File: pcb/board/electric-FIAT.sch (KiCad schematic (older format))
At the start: 25 parts, among them J1 Conn_01x10_Female, U4 OPA356xxDBV, U5 OPA356xxDBV, U6 STM32F405RGTx

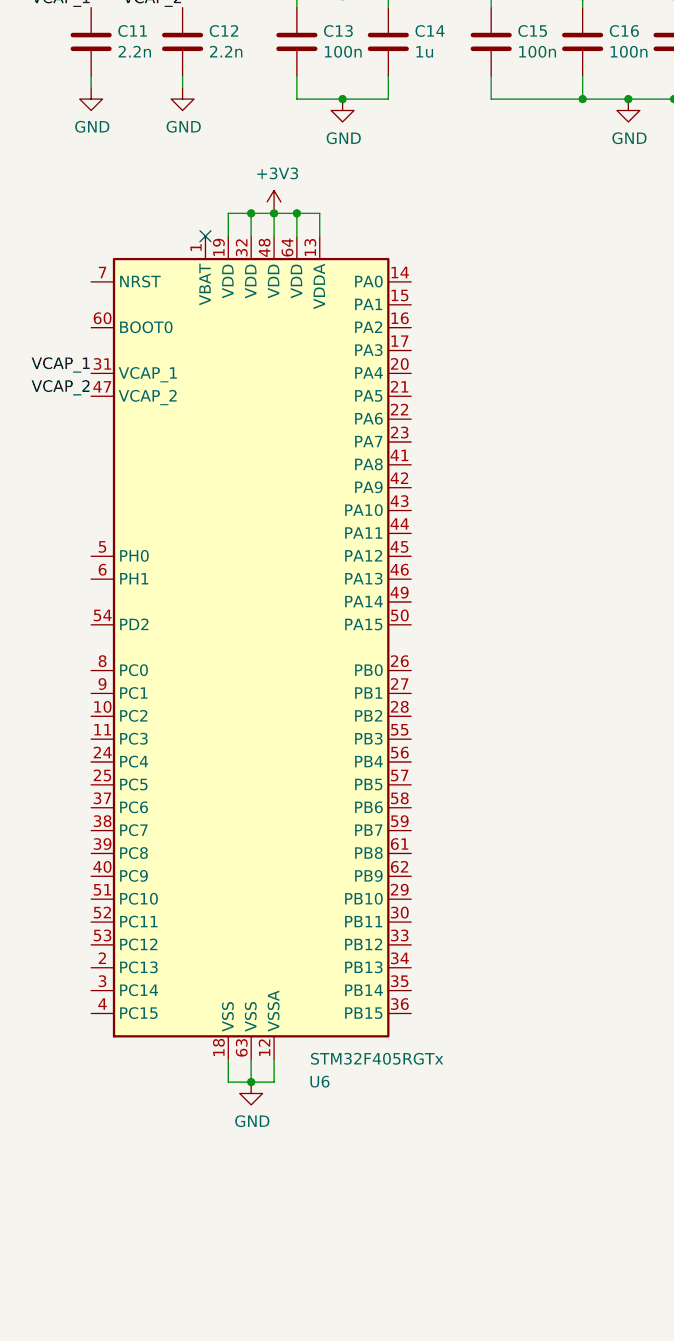
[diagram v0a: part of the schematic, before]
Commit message: Initialized STM32F405RGTx
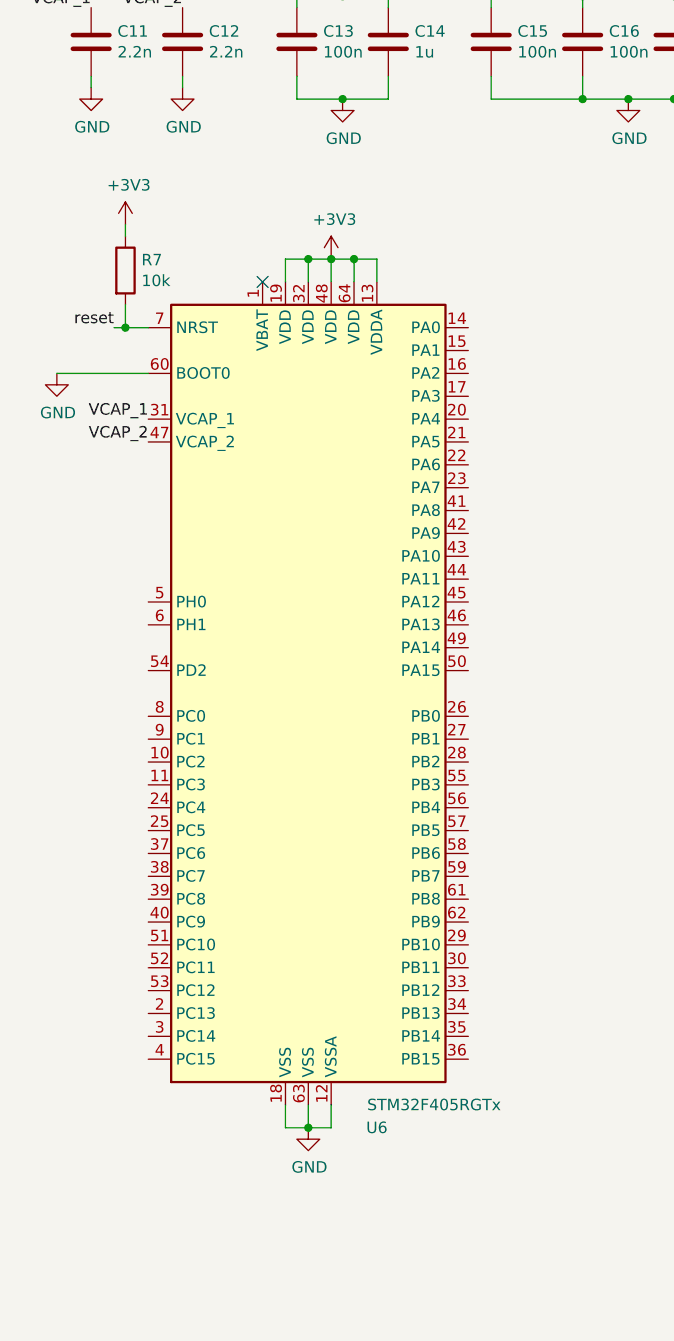
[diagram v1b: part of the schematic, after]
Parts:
- added R7: 10k, Resistor_SMD:R_0805_2012Metric, symbol Device:R
- J1: footprint (none) -> Connector_PinSocket_2.54mm:PinSocket_1x10_P2.54mm_Vertical
- TH1, TH2: footprint (none) -> TerminalBlock_RND:TerminalBlock_RND_205-00012_1x02_P5.00mm_Horizontal
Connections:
- net +3V3: now also R7.1
- net GND: now also U6.60 (BOOT0)
- net reset: now reaches U6.7 (NRST)
- net reset: now also R7.2
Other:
- moved on the sheet: U6
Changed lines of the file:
@@
 F 0 "TH1" H 7247 1746 50  0000 L CNN
 F 1 "KTY81" H 7247 1655 50  0000 L CNN
-F 2 "" V 7350 1700 50  0001 C CNN
+F 2 "TerminalBlock_RND:TerminalBlock_RND_205-00012_1x02_P5.00mm_Horizontal" V 7350 1700 50  0001 C CNN
 F 3 "http://www.nxp.com/documents/data_sheet/KTY81_SER.pdf" H 7150 1650 50  0001 C CNN
 	1    7150 1700
@@
 F 0 "TH2" H 9198 1746 50  0000 L CNN
 F 1 "Thermistor_NTC" H 9198 1655 50  0000 L CNN
-F 2 "" H 9100 1750 50  0001 C CNN
+F 2 "TerminalBlock_RND:TerminalBlock_RND_205-00012_1x02_P5.00mm_Horizontal" H 9100 1750 50  0001 C CNN
 F 3 "~" H 9100 1750 50  0001 C CNN
 	1    9100 1700
@@
 L MCU_ST_STM32F4:STM32F405RGTx U6
 U 1 1 5DC72DB0
-P 1550 3900
-F 0 "U6" H 1850 2000 50  0000 C CNN
-F 1 "STM32F405RGTx" H 2100 2100 50  0000 C CNN
-F 2 "Package_QFP:LQFP-64_10x10mm_P0.5mm" H 950 2200 50  0001 R CNN
-F 3 "http://www.st.com/st-web-ui/static/active/en/resource/technical/document/datasheet/DM00037051.pdf" H 1550 3900 50  0001 C CNN
-	1    1550 3900
+P 1800 4100
+F 0 "U6" H 2100 2200 50  0000 C CNN
+F 1 "STM32F405RGTx" H 2350 2300 50  0000 C CNN
+F 2 "Package_QFP:LQFP-64_10x10mm_P0.5mm" H 1200 2400 50  0001 R CNN
+F 3 "http://www.st.com/st-web-ui/static/active/en/resource/technical/document/datasheet/DM00037051.pdf" H 1800 4100 50  0001 C CNN
+	1    1800 4100
 	1    0    0    -1
 $EndComp
@@
 $EndComp
 Wire Wire Line
-	1550 2000 1450 2000
-Wire Wire Line
-	1550 2000 1550 2100
-Connection ~ 1550 2000
-Wire Wire Line
-	1450 2000 1450 2100
-Wire Wire Line
-	1650 2100 1650 2000
-Wire Wire Line
-	1650 2000 1550 2000
-Wire Wire Line
-	1750 2100 1750 2000
-Wire Wire Line
-	1750 2000 1650 2000
-Connection ~ 1650 2000
-Wire Wire Line
-	1850 2100 1850 2000
-Wire Wire Line
-	1850 2000 1750 2000
-Connection ~ 1750 2000
+	1800 2200 1700 2200
+Wire Wire Line
+	1800 2200 1800 2300
+Connection ~ 1800 2200
+Wire Wire Line
+	1700 2200 1700 2300
+Wire Wire Line
+	1900 2300 1900 2200
+Wire Wire Line
+	1900 2200 1800 2200
+Wire Wire Line
+	2000 2300 2000 2200
+Wire Wire Line
+	2000 2200 1900 2200
+Connection ~ 1900 2200
+Wire Wire Line
+	2100 2300 2100 2200
+Wire Wire Line
+	2100 2200 2000 2200
+Connection ~ 2000 2200
 $Comp
 L power:GND #PWR027
 U 1 1 5DC7D7B5
-P 1550 5800
-F 0 "#PWR027" H 1550 5550 50  0001 C CNN
-F 1 "GND" H 1555 5627 50  0000 C CNN
-F 2 "" H 1550 5800 50  0001 C CNN
-F 3 "" H 1550 5800 50  0001 C CNN
-	1    1550 5800
-	1    0    0    -1
-$EndComp
-Wire Wire Line
-	1550 5800 1450 5800
-Wire Wire Line
-	1450 5800 1450 5700
-Wire Wire Line
-	1550 5700 1550 5800
-Connection ~ 1550 5800
-Wire Wire Line
-	1650 5700 1650 5800
-Wire Wire Line
-	1650 5800 1550 5800
+P 1800 6000
+F 0 "#PWR027" H 1800 5750 50  0001 C CNN
+F 1 "GND" H 1805 5827 50  0000 C CNN
+F 2 "" H 1800 6000 50  0001 C CNN
+F 3 "" H 1800 6000 50  0001 C CNN
+	1    1800 6000
+	1    0    0    -1
+$EndComp
+Wire Wire Line
+	1800 6000 1700 6000
+Wire Wire Line
+	1700 6000 1700 5900
+Wire Wire Line
+	1800 5900 1800 6000
+Connection ~ 1800 6000
+Wire Wire Line
+	1900 5900 1900 6000
+Wire Wire Line
+	1900 6000 1800 6000
 $Comp
 L Device:C C12
@@
 	1    0    0    -1
 $EndComp
-Text Label 850  2700 2    50   ~ 0
+Text Label 1100 2900 2    50   ~ 0
 VCAP_1
-Text Label 850  2800 2    50   ~ 0
+Text Label 1100 3000 2    50   ~ 0
 VCAP_2
 Text Label 850  1100 2    50   ~ 0
@@
 Text Notes 1700 1000 0    50   ~ 0
 ADC
-NoConn ~ 1350 2100
+NoConn ~ 1600 2300
 $Comp
 L Device:C C15
@@
 L power:+3V3 #PWR034
 U 1 1 5DCEBEA8
-P 1650 2000
-F 0 "#PWR034" H 1650 1850 50  0001 C CNN
-F 1 "+3V3" H 1665 2173 50  0000 C CNN
-F 2 "" H 1650 2000 50  0001 C CNN
-F 3 "" H 1650 2000 50  0001 C CNN
-	1    1650 2000
+P 1900 2200
+F 0 "#PWR034" H 1900 2050 50  0001 C CNN
+F 1 "+3V3" H 1915 2373 50  0000 C CNN
+F 2 "" H 1900 2200 50  0001 C CNN
+F 3 "" H 1900 2200 50  0001 C CNN
+	1    1900 2200
 	1    0    0    -1
 $EndComp
@@
 F 0 "J1" H 6028 6976 50  0000 L CNN
 F 1 "Conn_01x10_Female" H 6028 6885 50  0000 L CNN
-F 2 "" H 6000 7000 50  0001 C CNN
+F 2 "Connector_PinSocket_2.54mm:PinSocket_1x10_P2.54mm_Vertical" H 6000 7000 50  0001 C CNN
 F 3 "~" H 6000 7000 50  0001 C CNN
 	1    6000 7000
@@
 	5100 6700 5800 6700
 Connection ~ 5100 7000
+$Comp
+L power:GND #PWR041
+U 1 1 5DD53313
+P 700 2700
+F 0 "#PWR041" H 700 2450 50  0001 C CNN
+F 1 "GND" H 705 2527 50  0000 C CNN
+F 2 "" H 700 2700 50  0001 C CNN
+F 3 "" H 700 2700 50  0001 C CNN
+	1    700  2700
+	1    0    0    -1
+$EndComp
+Wire Wire Line
+	700  2700 1100 2700
+Text Label 950  2500 2    50   ~ 0
+reset
+$Comp
+L power:+3V3 #PWR040
+U 1 1 5DD5B29D
+P 1000 2050
+F 0 "#PWR040" H 1000 1900 50  0001 C CNN
+F 1 "+3V3" H 1015 2223 50  0000 C CNN
+F 2 "" H 1000 2050 50  0001 C CNN
+F 3 "" H 1000 2050 50  0001 C CNN
+	1    1000 2050
+	1    0    0    -1
+$EndComp
+$Comp
+L Device:R R7
+U 1 1 5DD5BE82
+P 1000 2250
+F 0 "R7" H 1070 2296 50  0000 L CNN
+F 1 "10k" H 1070 2205 50  0000 L CNN
+F 2 "Resistor_SMD:R_0805_2012Metric" V 930 2250 50  0001 C CNN
+F 3 "~" H 1000 2250 50  0001 C CNN
+	1    1000 2250
+	1    0    0    -1
+$EndComp
+Wire Wire Line
+	1000 2050 1000 2100
+Wire Wire Line
+	950  2500 1000 2500
+Wire Wire Line
+	1000 2400 1000 2500
+Connection ~ 1000 2500
+Wire Wire Line
+	1000 2500 1100 2500
 $EndSCHEMATC
